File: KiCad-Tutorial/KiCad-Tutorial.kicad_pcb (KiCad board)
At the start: 4 copper layers, 23.2 x 51.1 mm, 10 parts, among them J1 Conn_01x20_Pin, J2 Conn_01x20_Pin, J3 USB_B_Micro, SW1 SW_MEC_5E, SW2 SW_MEC_5E, U1 TLV75801PDRV, U2 ESP32-S3-MINI-1, U3 D3V3XA4B10LP

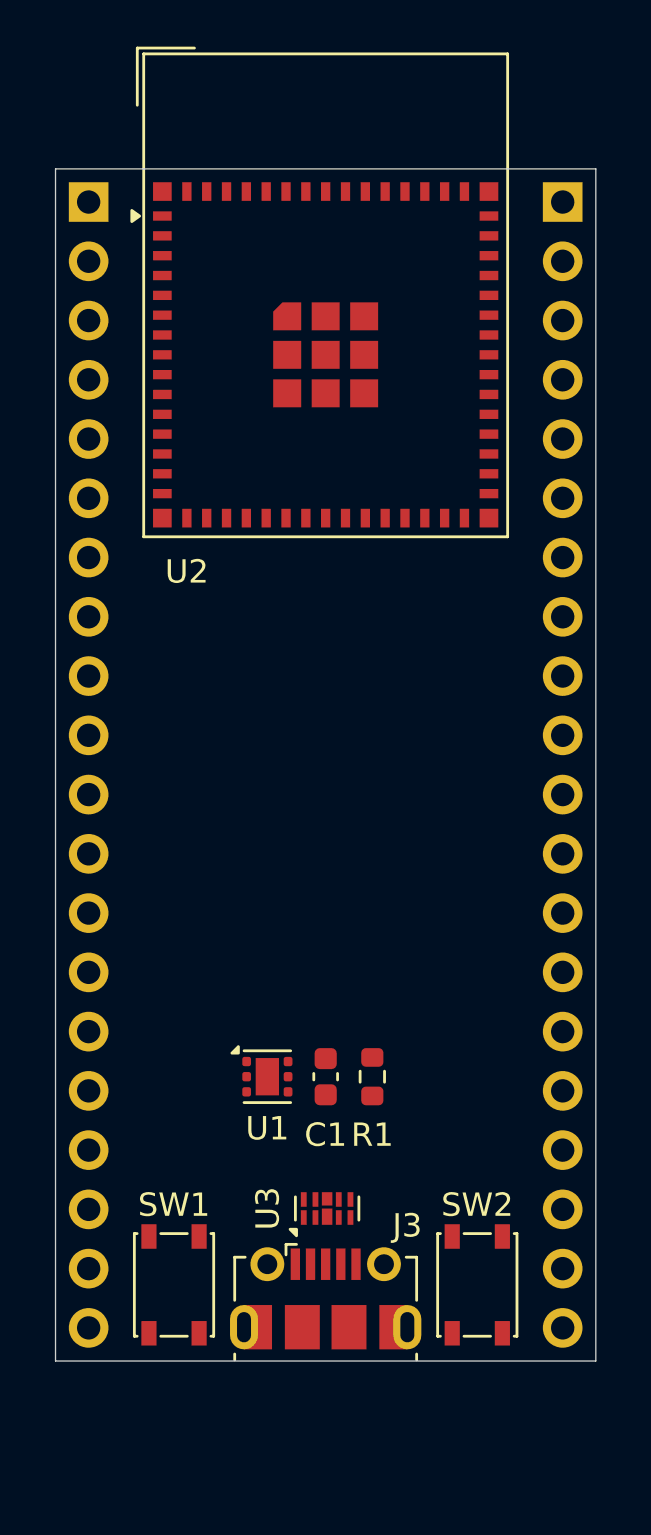
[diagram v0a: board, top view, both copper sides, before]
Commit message: Example Done
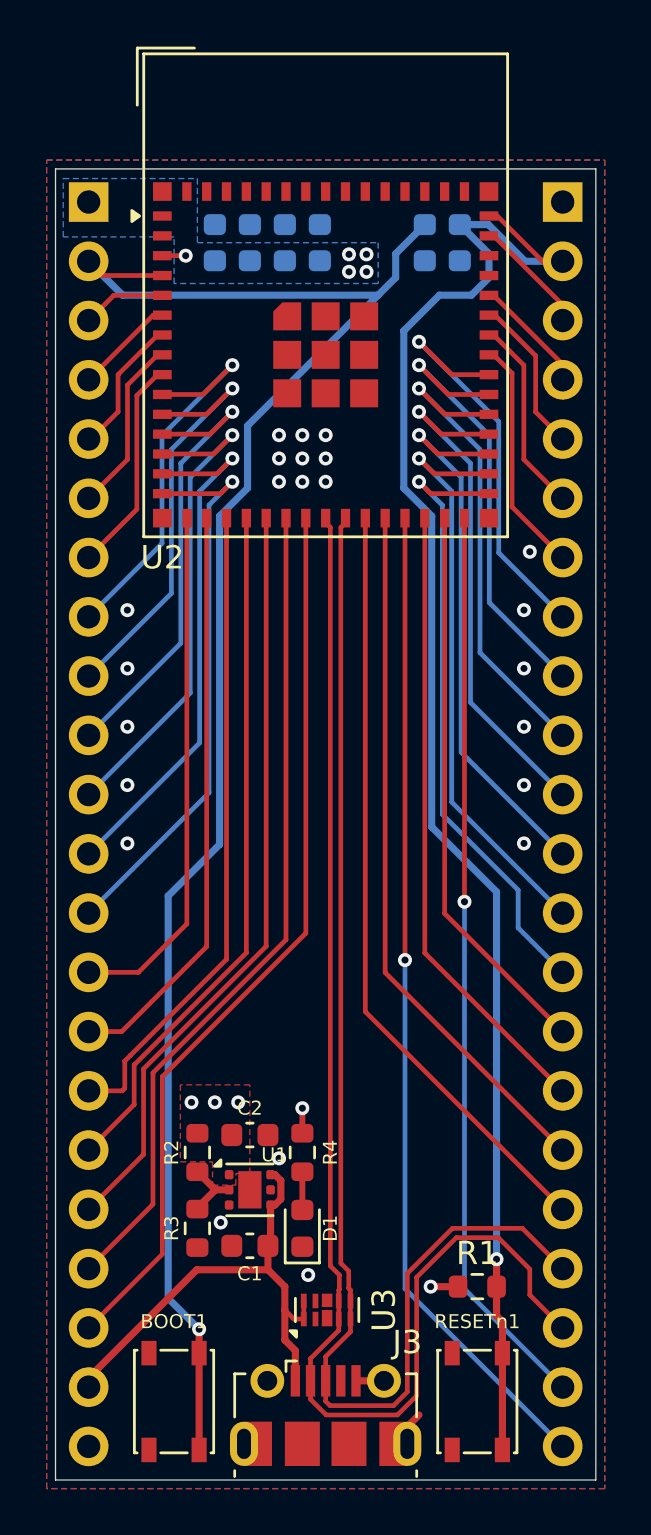
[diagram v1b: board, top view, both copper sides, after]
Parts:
- added C2: 10uF, Capacitor_SMD:C_0603_1608Metric, F.Cu at (116.8, 113.0)
- added C3: 0.1uF, Capacitor_SMD:C_0603_1608Metric, B.Cu at (125.8, 74.8)
- added C4: 0.1uF, Capacitor_SMD:C_0603_1608Metric, B.Cu at (124.2, 74.8)
- added C5: 10uF, Capacitor_SMD:C_0603_1608Metric, B.Cu at (119.8, 74.8)
- added C6: 10uF, Capacitor_SMD:C_0603_1608Metric, B.Cu at (118.2, 74.8)
- added C7: 0.1uF, Capacitor_SMD:C_0603_1608Metric, B.Cu at (116.8, 74.8)
- added C8: 0.1uF, Capacitor_SMD:C_0603_1608Metric, B.Cu at (115.2, 74.8)
- added D1: LED, LED_SMD:LED_0603_1608Metric, F.Cu at (119.0, 117.0)
- added G***: LOGO, LOGO, B.Cu at (120.0, 91.0)
- added R2: 1M, Resistor_SMD:R_0603_1608Metric, F.Cu at (114.5, 113.8)
- added R3: 200k, Resistor_SMD:R_0603_1608Metric, F.Cu at (114.5, 117.0)
- added R4: 330, Resistor_SMD:R_0603_1608Metric, F.Cu at (119.0, 113.8)
- C1: value C -> 10uF
- J1, J2: value Conn_01x20_Pin -> Conn_01x22_Pin; footprint Connector_PinHeader_2.54mm:PinHeader_1x20_P2.54mm_Vertical -> Connector_PinHeader_2.54mm:PinHeader_1x22_P2.54mm_Vertical
- R1: value R -> 10k
- moved R1 10.1 mm to (126.5, 119.5), turned to 0 degrees
- moved C1 7.95 mm to (116.8, 117.8), turned to 180 degrees
- moved BOOT1 5.00 mm to (113.5, 124.4)
- moved J3 5.00 mm to (120.0, 125.0)
- moved RESETn1 5.00 mm to (126.5, 124.4)
- moved U1 4.91 mm to (116.8, 115.3)
- moved U3 4.35 mm to (120.1, 120.5)
- renumbered SW1 to BOOT1, SW2 to RESETn1
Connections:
- BOOT1 pad 1: unconnected-(SW1-Pad1) -> GND
- BOOT1 pad 2: unconnected-(SW1-Pad2) -> GND
- BOOT1 pad 3: unconnected-(SW1-K-Pad3) -> /BOOT
- BOOT1 pad 4: unconnected-(SW1-A-Pad4) -> /BOOT
- C1 pad 1: unconnected-(C1-Pad1) -> /USB_5V
- C1 pad 2: unconnected-(C1-Pad2) -> GND
- J1 pad 1: unconnected-(J1-Pin_1-Pad1) -> +3.3V
- J1 pad 10: unconnected-(J1-Pin_10-Pad10) -> /IO8
- J1 pad 11: unconnected-(J1-Pin_11-Pad11) -> /IO9
- J1 pad 12: unconnected-(J1-Pin_12-Pad12) -> /IO10
- J1 pad 13: unconnected-(J1-Pin_13-Pad13) -> /IO11
- J1 pad 14: unconnected-(J1-Pin_14-Pad14) -> /IO12
- J1 pad 15: unconnected-(J1-Pin_15-Pad15) -> /IO13
- J1 pad 16: unconnected-(J1-Pin_16-Pad16) -> /IO14
- J1 pad 17: unconnected-(J1-Pin_17-Pad17) -> /IO15
- J1 pad 18: unconnected-(J1-Pin_18-Pad18) -> /IO16
- J1 pad 19: unconnected-(J1-Pin_19-Pad19) -> /IO17
- J1 pad 2: unconnected-(J1-Pin_2-Pad2) -> /BOOT
- J1 pad 20: unconnected-(J1-Pin_20-Pad20) -> /IO18
- J1 pad 3: unconnected-(J1-Pin_3-Pad3) -> /IO1
- J1 pad 4: unconnected-(J1-Pin_4-Pad4) -> /IO2
- J1 pad 5: unconnected-(J1-Pin_5-Pad5) -> /IO3
- J1 pad 6: unconnected-(J1-Pin_6-Pad6) -> /IO4
- J1 pad 7: unconnected-(J1-Pin_7-Pad7) -> /IO5
- J1 pad 8: unconnected-(J1-Pin_8-Pad8) -> /IO6
- J1 pad 9: unconnected-(J1-Pin_9-Pad9) -> /IO7
- J2 pad 1: unconnected-(J2-Pin_1-Pad1) -> GND
- J2 pad 10: unconnected-(J2-Pin_10-Pad10) -> /IO39
- J2 pad 11: unconnected-(J2-Pin_11-Pad11) -> /IO38
- J2 pad 12: unconnected-(J2-Pin_12-Pad12) -> /IO37
- J2 pad 13: unconnected-(J2-Pin_13-Pad13) -> /IO36
- J2 pad 14: unconnected-(J2-Pin_14-Pad14) -> /IO35
- J2 pad 15: unconnected-(J2-Pin_15-Pad15) -> /IO34
- J2 pad 16: unconnected-(J2-Pin_16-Pad16) -> /IO33
- J2 pad 17: unconnected-(J2-Pin_17-Pad17) -> /IO26
- J2 pad 18: unconnected-(J2-Pin_18-Pad18) -> /IO21
- J2 pad 19: unconnected-(J2-Pin_19-Pad19) -> /USB_D+
- J2 pad 2: unconnected-(J2-Pin_2-Pad2) -> /RSTn
- J2 pad 20: unconnected-(J2-Pin_20-Pad20) -> /USB_D-
- J2 pad 3: unconnected-(J2-Pin_3-Pad3) -> /IO46
- J2 pad 4: unconnected-(J2-Pin_4-Pad4) -> /IO45
- J2 pad 5: unconnected-(J2-Pin_5-Pad5) -> /RXD0
- J2 pad 6: unconnected-(J2-Pin_6-Pad6) -> /TXD0
- J2 pad 7: unconnected-(J2-Pin_7-Pad7) -> /IO42
- J2 pad 8: unconnected-(J2-Pin_8-Pad8) -> /IO41
- J2 pad 9: unconnected-(J2-Pin_9-Pad9) -> /IO40
- J3 pad 1: unconnected-(J3-VBUS-Pad1) -> /USB_5V
- J3 pad 2: unconnected-(J3-D--Pad2) -> /USB_D-
- J3 pad 3: unconnected-(J3-D+-Pad3) -> /USB_D+
- J3 pad 5: unconnected-(J3-GND-Pad5) -> GND
- J3 pad 6: unconnected-(J3-Shield-Pad6) -> GND
- R1 pad 1: unconnected-(R1-Pad1) -> +3.3V
- R1 pad 2: unconnected-(R1-Pad2) -> /RSTn
- RESETn1 pad 1: unconnected-(SW2-Pad1) -> GND
- RESETn1 pad 2: unconnected-(SW2-Pad2) -> GND
- RESETn1 pad 3: unconnected-(SW2-K-Pad3) -> /RSTn
- RESETn1 pad 4: unconnected-(SW2-A-Pad4) -> /RSTn
- U1 pad 1: unconnected-(U1-OUT-Pad1) -> +3.3V
- U1 pad 2: unconnected-(U1-FB-Pad2) -> Net-(U1-FB)
- U1 pad 3: Net-(U1-GND-Pad3) -> GND
- U1 pad 4: unconnected-(U1-EN-Pad4) -> /USB_5V
- U1 pad 6: unconnected-(U1-IN-Pad6) -> /USB_5V
- U1 pad 7: Net-(U1-GND-Pad3) -> GND
- U2 pad 10: unconnected-(U2-IO6-Pad10) -> /IO6
- U2 pad 11: unconnected-(U2-IO7-Pad11) -> /IO7
- U2 pad 12: unconnected-(U2-IO8-Pad12) -> /IO8
- U2 pad 13: unconnected-(U2-IO9-Pad13) -> /IO9
- U2 pad 14: unconnected-(U2-IO10-Pad14) -> /IO10
- U2 pad 15: unconnected-(U2-IO11-Pad15) -> /IO11
- U2 pad 16: unconnected-(U2-IO12-Pad16) -> /IO12
- U2 pad 17: unconnected-(U2-IO13-Pad17) -> /IO13
- U2 pad 18: unconnected-(U2-IO14-Pad18) -> /IO14
- U2 pad 19: unconnected-(U2-IO15-Pad19) -> /IO15
- U2 pad 20: unconnected-(U2-IO16-Pad20) -> /IO16
- U2 pad 21: unconnected-(U2-IO17-Pad21) -> /IO17
- U2 pad 22: unconnected-(U2-IO18-Pad22) -> /IO18
- U2 pad 23: unconnected-(U2-USB_D--Pad23) -> /USB_D-
- U2 pad 24: unconnected-(U2-USB_D+-Pad24) -> /USB_D+
- U2 pad 25: unconnected-(U2-IO21-Pad25) -> /IO21
- U2 pad 26: unconnected-(U2-IO26-Pad26) -> /IO26
- U2 pad 27: unconnected-(U2-IO47-Pad27) -> /IO47
- U2 pad 28: unconnected-(U2-IO33-Pad28) -> /IO33
- U2 pad 29: unconnected-(U2-IO34-Pad29) -> /IO34
- U2 pad 3: unconnected-(U2-3V3-Pad3) -> +3.3V
- U2 pad 30: unconnected-(U2-IO48-Pad30) -> /IO48
- U2 pad 31: unconnected-(U2-IO35-Pad31) -> /IO35
- U2 pad 32: unconnected-(U2-IO36-Pad32) -> /IO36
- U2 pad 33: unconnected-(U2-IO37-Pad33) -> /IO37
- U2 pad 34: unconnected-(U2-IO38-Pad34) -> /IO38
- U2 pad 35: unconnected-(U2-IO39-Pad35) -> /IO39
- U2 pad 36: unconnected-(U2-IO40-Pad36) -> /IO40
- U2 pad 37: unconnected-(U2-IO41-Pad37) -> /IO41
- U2 pad 38: unconnected-(U2-IO42-Pad38) -> /IO42
- U2 pad 39: unconnected-(U2-TXD0-Pad39) -> /TXD0
- U2 pad 4: unconnected-(U2-IO0-Pad4) -> /BOOT
- U2 pad 40: unconnected-(U2-RXD0-Pad40) -> /RXD0
- U2 pad 41: unconnected-(U2-IO45-Pad41) -> /IO45
- U2 pad 44: unconnected-(U2-IO46-Pad44) -> /IO46
- U2 pad 45: unconnected-(U2-EN-Pad45) -> /RSTn
- U2 pad 5: unconnected-(U2-IO1-Pad5) -> /IO1
- U2 pad 6: unconnected-(U2-IO2-Pad6) -> /IO2
- U2 pad 7: unconnected-(U2-IO3-Pad7) -> /IO3
- U2 pad 8: unconnected-(U2-IO4-Pad8) -> /IO4
- U2 pad 9: unconnected-(U2-IO5-Pad9) -> /IO5
- U3 pad 1: unconnected-(U3-Pad1) -> /USB_5V
- U3 pad 10: unconnected-(U3-NC-Pad10) -> /USB_5V
- U3 pad 3: Net-(U3-VSS-Pad3) -> GND
- U3 pad 4: unconnected-(U3-Pad4) -> /USB_D-
- U3 pad 5: unconnected-(U3-Pad5) -> /USB_D+
- U3 pad 6: unconnected-(U3-NC-Pad6) -> /USB_D+
- U3 pad 7: unconnected-(U3-NC-Pad7) -> /USB_D-
- U3 pad 8: Net-(U3-VSS-Pad3) -> GND
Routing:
- net /BOOT: track 0.00 -> 74.1 mm, vias 0 -> 1
- net /RSTn: track 0.00 -> 66.1 mm, vias 0 -> 1
- net /USB_D-: track 0.00 -> 58.0 mm
- net /USB_D+: track 0.00 -> 55.6 mm
- net /IO47: track 0.00 -> 42.6 mm, vias 0 -> 1
- net /IO48: track 0.00 -> 39.0 mm, vias 0 -> 1
- net /IO18: track 0.00 -> 38.6 mm
- net /IO17: track 0.00 -> 35.7 mm
- net /IO21: track 0.00 -> 33.1 mm
- net /IO16: track 0.00 -> 32.8 mm
- net /IO26: track 0.00 -> 30.2 mm
- net /IO15: track 0.00 -> 29.9 mm
- net /IO14: track 0.00 -> 27.8 mm
- net /IO33: track 0.00 -> 27.0 mm
- net /IO35: track 0.00 -> 26.8 mm, vias 0 -> 1
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- added copper zone on B.Cu, net +3.3V
- added copper zone on F.Cu, net +3.3V
- added copper zone on In1.Cu, net +3.3V
- added copper zone on B.Cu, net GND
- added copper zone on F.Cu, net GND
- added copper zone on In2.Cu, net GND
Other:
- board size 23.2 x 51.1 mm -> 23.2 x 56.2 mm
- board text added: "CPP DIGITAL Hardware Design Team ESP32 Intro Dev Board Designer: Max Gross Date: 3/2/2025"
- board text removed: "CPP DIGITAL Hardware Design Team ESP32 Intro Dev Board Designer: [Your Name Here!] Date: 3/2/2025"
